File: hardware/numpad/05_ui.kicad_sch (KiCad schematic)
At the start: 5 parts, among them J3 Conn_01x04, Q1 BSS138, Q2 BSS138

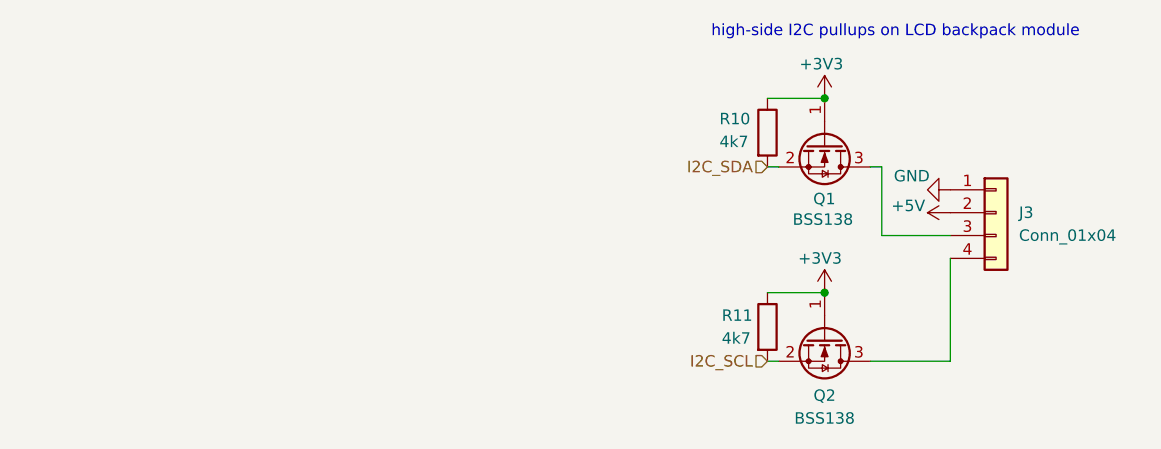
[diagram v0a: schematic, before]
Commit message: Format cleanup, titles
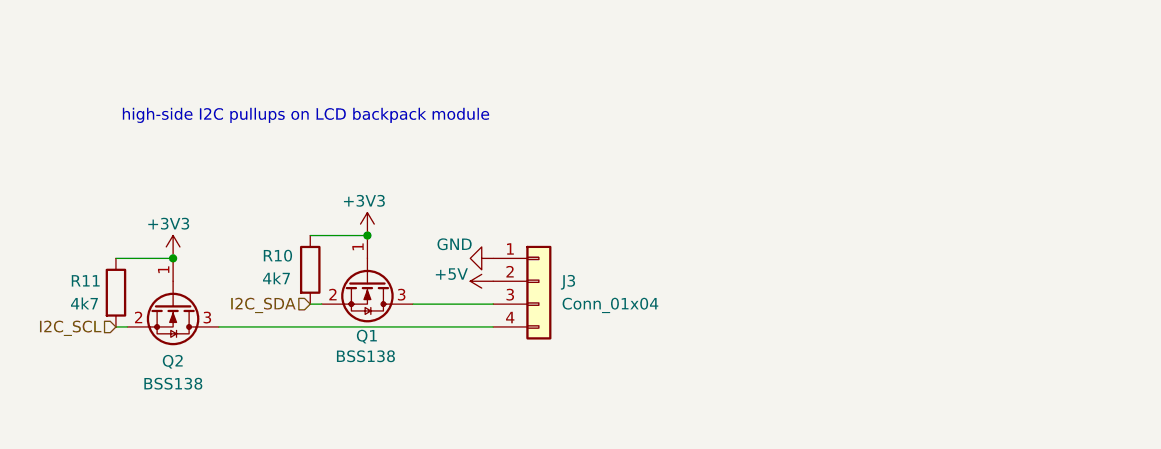
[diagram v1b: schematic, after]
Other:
- title: (none) -> LCD I2C Connectors
- moved on the sheet: J3, Q1, Q2, R10, R11

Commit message: footprints set
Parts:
- J3: footprint (none) -> Connector_PinHeader_2.54mm:PinHeader_1x04_P2.54mm_Vertical
- R10, R11: footprint (none) -> Resistor_SMD:R_0603_1608Metric
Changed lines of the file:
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@@
 			)
 		)
-		(property "Footprint" ""
+		(property "Footprint" "Resistor_SMD:R_0603_1608Metric"
 			(at 74.422 64.77 90)
 			(hide yes)
@@
 			)
 		)
-		(property "Footprint" ""
+		(property "Footprint" "Resistor_SMD:R_0603_1608Metric"
 			(at 96.012 62.23 90)
 			(hide yes)
@@
 			)
 		)
-		(property "Footprint" ""
+		(property "Footprint" "Connector_PinHeader_2.54mm:PinHeader_1x04_P2.54mm_Vertical"
 			(at 123.19 63.5 0)
 			(hide yes)
